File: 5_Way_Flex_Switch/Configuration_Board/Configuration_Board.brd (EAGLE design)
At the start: 17.8 x 5 mm, 1 part

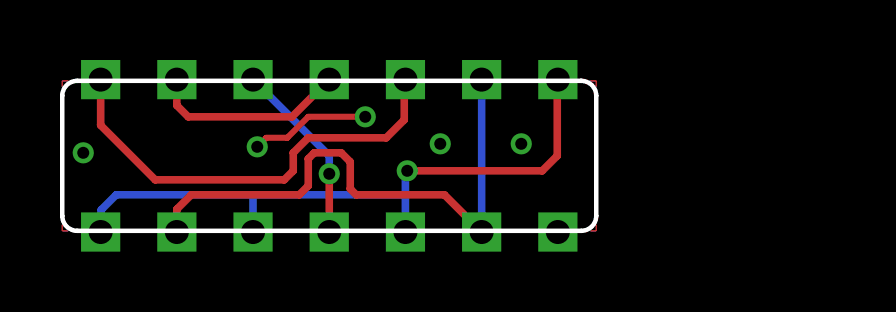
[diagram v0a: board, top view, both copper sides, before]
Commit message: Licenses
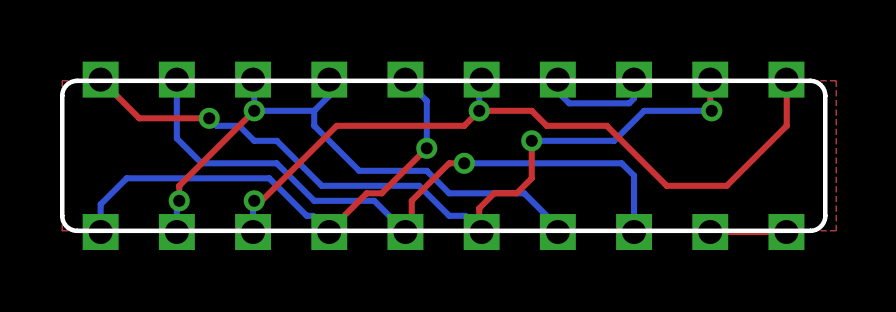
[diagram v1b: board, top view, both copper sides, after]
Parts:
- removed U$1: CONFIGURATION_BRD_, CYCFI_Module_castellated:CONFIGURATION_BRD_MOD
- added CB1: (no value), CYCFI_Module_castellated:CONFIGURATION_BRD_CAST
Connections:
- removed net B1: U$1.3-OC, U$1.B1
- removed net IN-: U$1.1-IC, U$1.3-IC, U$1.4-IC, U$1.IN-
- removed net M1: U$1.2-OC, U$1.M1
- removed net N1: U$1.1-OC, U$1.N1
- removed net N2: U$1.2-IC, U$1.4-OC, U$1.N2
- new net 1: CB1.3-OC, CB1.N1, CB1.OUT+
- new net 2: CB1.3-IC, CB1.4-OC, CB1.M1
- new net 3: CB1.1-OC, CB1.4-IC, CB1.B1, CB1.N2
- new net 4: CB1.COM1, CB1.COM2
- new net 5: CB1.1-IC, CB1.2-OC, CB1.M2
- new net 6: CB1.2-IC, CB1.B2, CB1.OUT-
- net GND: now also CB1.GND, CB1.GND1; no longer U$1.GND
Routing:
- net 1: track 0.00 -> 26.5 mm, vias 0 -> 3
- net 6: track 0.00 -> 24.5 mm, vias 0 -> 2
- net IN-: track 22.2 -> 0.00 mm, vias 1 -> 0
- net 2: track 0.00 -> 22.0 mm, vias 0 -> 1
- net 3: track 0.00 -> 19.6 mm, vias 0 -> 2
- net N2: track 18.9 -> 0.00 mm
- net 5: track 0.00 -> 16.7 mm, vias 0 -> 1
- net N1: track 14.9 -> 0.00 mm
- net M1: track 6.61 -> 0.00 mm
- net B1: track 6.13 -> 0.00 mm, vias 1 -> 0
- net 4: track 0.00 -> 3.80 mm
- net GND: track 4.01 -> 2.54 mm, vias 5 -> 0
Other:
- board size 17.8 x 5 mm -> 25.4 x 5 mm
